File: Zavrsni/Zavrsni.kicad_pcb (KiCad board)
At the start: 2 copper layers, 104 x 58.3 mm, 23 parts, among them J1 12V Source, J3 Output A, J5 Conn_01x04, J6 Conn_02x19_Odd_Even, J7 Conn_02x19_Odd_Even, J8 Conn_01x06, U1 LM78M05_TO220, U2 L298N

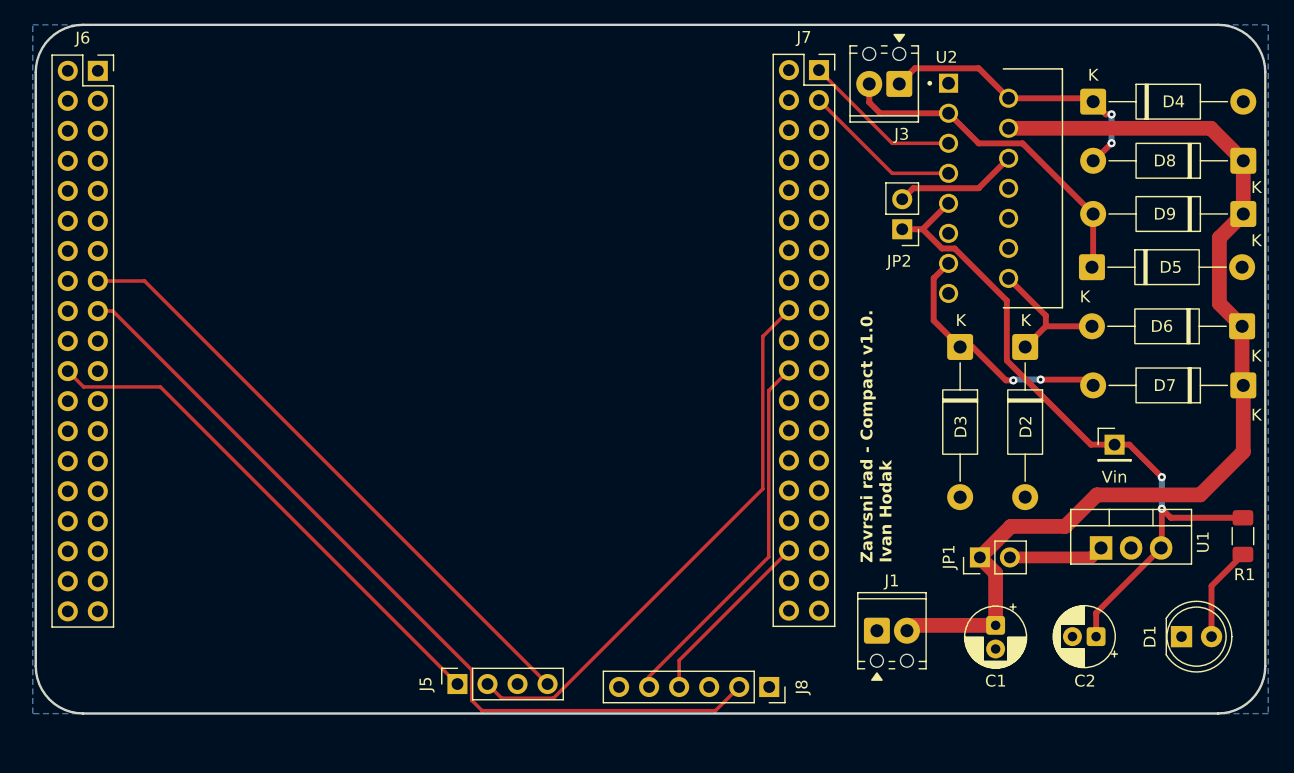
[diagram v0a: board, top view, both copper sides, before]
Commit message: update
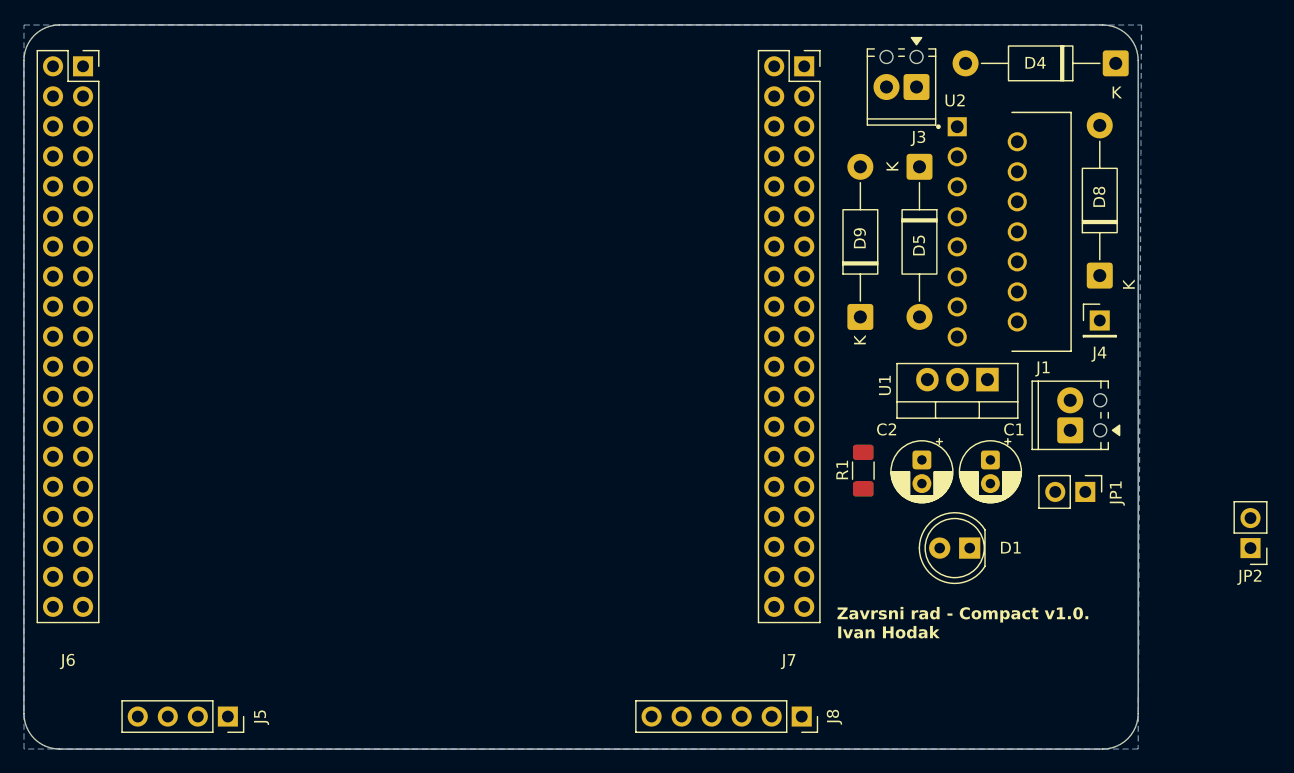
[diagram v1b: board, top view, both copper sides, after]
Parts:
- removed D2, D3, D6, D7: D_Schottky_Filled, Diode_THT:D_DO-41_SOD81_P12.70mm_Horizontal
- moved JP2 39.9 mm to (223.8, 125.8)
- moved D9 33.5 mm to (190.8, 106.2), turned to 90 degrees
- moved R1 32.6 mm to (191.0, 119.2)
- moved J1 23.6 mm to (208.5, 115.8), turned to 90 degrees
- moved C2 21.0 mm to (196.0, 118.3), turned to -90 degrees
- moved J5 19.6 mm to (137.2, 140.0), turned to -90 degrees
- moved D1 19.4 mm to (200.0, 125.8), turned to 180 degrees
- moved U1 17.2 mm to (201.5, 111.5), turned to 180 degrees
- moved D5 16.9 mm to (195.8, 93.5), turned to -90 degrees
- moved D8 15.5 mm to (211.0, 102.7), turned to 90 degrees
- moved C1 14.0 mm to (201.8, 118.3)
- moved J4 10.6 mm to (211.0, 106.5)
- moved JP1 10.5 mm to (209.8, 121.0), turned to -90 degrees
- moved D4 3.76 mm to (212.3, 84.8), turned to 180 degrees
- moved U2 3.75 mm to (198.9, 90.1)
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- renumbered Vin to J4
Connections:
- U2 pad 13: Net-(D3-K) -> unconnected-(U2-OUT3-Pad13)
- U2 pad 14: Net-(D2-K) -> unconnected-(U2-OUT4-Pad14)
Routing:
- net 12V: track 87.3 -> 0.00 mm
- net 5V BL: track 70.6 -> 0.00 mm
- net 5V: track 59.7 -> 0.00 mm, vias 2 -> 0
- net 3V3: track 52.2 -> 0.00 mm
- net SCL: track 47.1 -> 0.00 mm
- net SDA: track 43.9 -> 0.00 mm
- net RX: track 31.7 -> 0.00 mm
- net OUT2: track 28.9 -> 0.00 mm
- net OUT1: track 24.7 -> 0.00 mm, vias 2 -> 0
- net Net-(D3-K): track 21.2 -> 0.00 mm, vias 2 -> 0
- net TX: track 15.4 -> 0.00 mm
- net IN1: track 13.5 -> 0.00 mm
- net IN2: track 13.5 -> 0.00 mm
- net Net-(D2-K): track 11.7 -> 0.00 mm
- net Net-(JP2-B): track 10.4 -> 0.00 mm
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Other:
- board size 104 x 58.3 mm -> 94.2 x 61.2 mm
